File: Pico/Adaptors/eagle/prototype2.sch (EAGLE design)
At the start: 13 parts, among them J1 JST-2P-SMD-PW-3410050P1

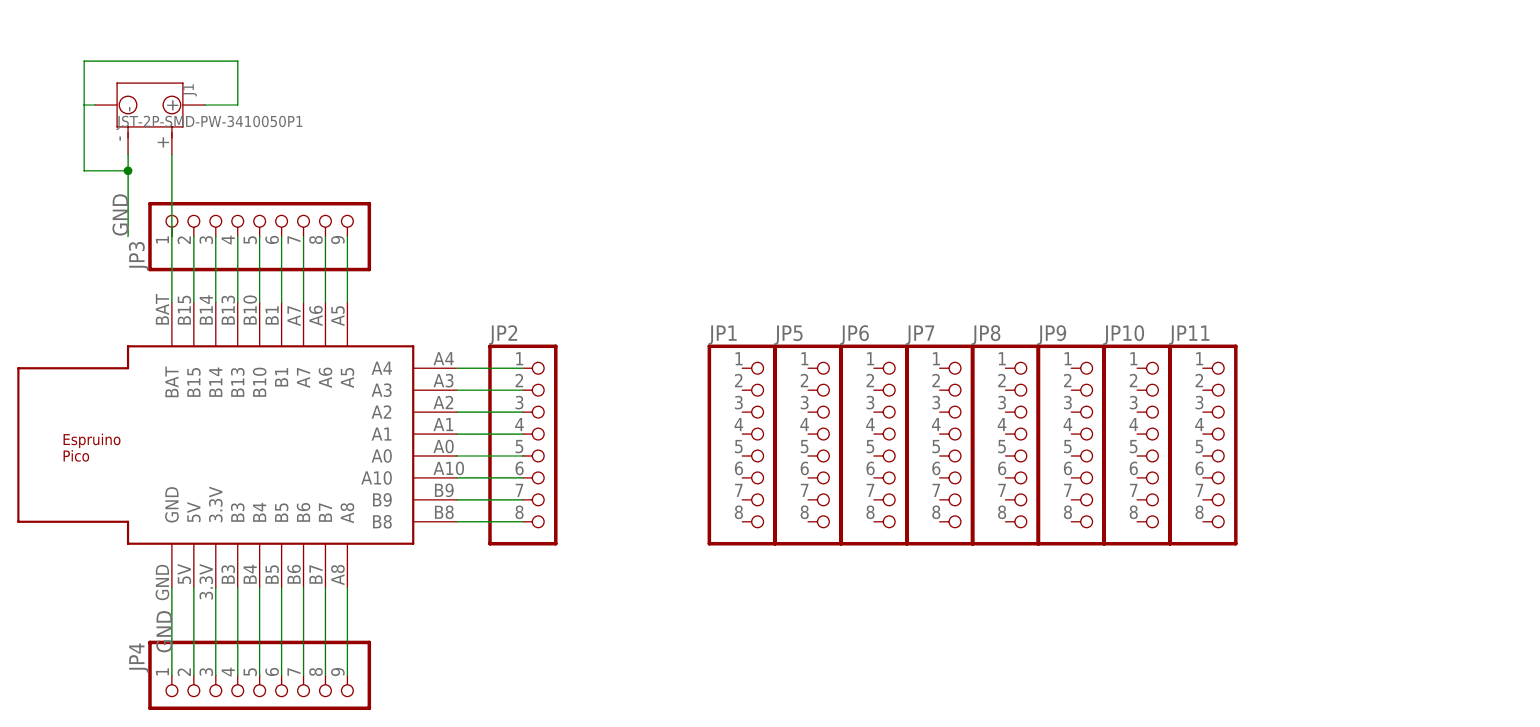
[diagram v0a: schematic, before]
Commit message: a full panel
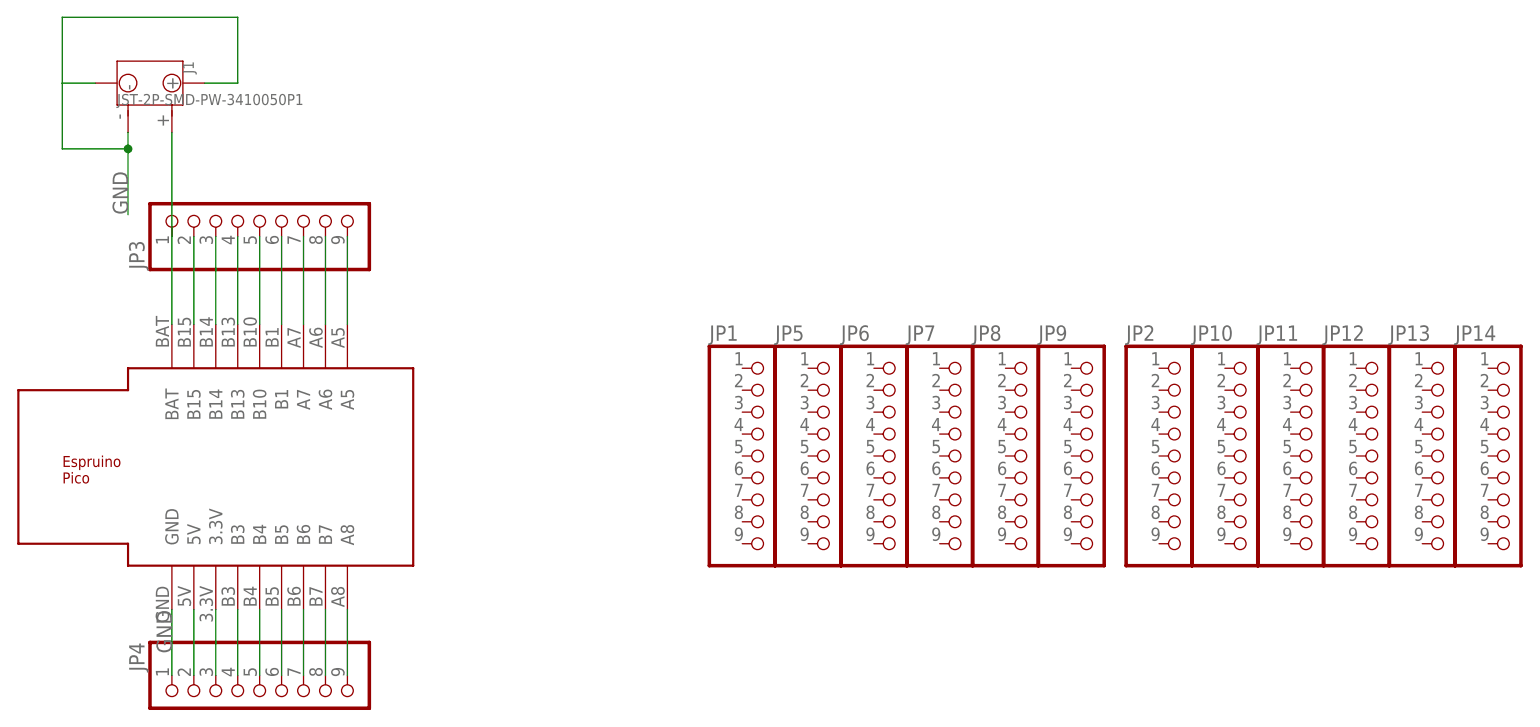
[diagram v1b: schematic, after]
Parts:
- added JP12, JP13, JP14: (no value), pinhead-2:PINHD-1X09_2.54-S
- JP1, JP10, JP11, JP2, JP5, JP6, JP7, JP8, JP9: device pinhead-2:PINHD-1X08_2.54-S -> pinhead-2:PINHD-1X09_2.54-S
- U$1: value ESPRUINO_PICO_SMD -> ESPRUINO_PICO_0.1; device espruino_pico:ESPRUINO_PICO_SMD -> espruino_pico:ESPRUINO_PICO_0.1
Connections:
- removed net N$1: JP2.2, U$1.A3
- removed net N$2: JP2.3, U$1.A2
- removed net N$24: JP2.1, U$1.A4
- removed net N$3: JP2.4, U$1.A1
- removed net N$4: JP2.5, U$1.A0
- removed net N$5: JP2.6, U$1.A10
- removed net N$6: JP2.7, U$1.B9
- removed net N$9: JP2.8, U$1.B8
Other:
- moved on the sheet: J1
